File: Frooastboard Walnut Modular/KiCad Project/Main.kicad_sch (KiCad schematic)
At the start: 322 parts, among them J12 Conn_01x16, J13 Conn_01x06, J14 Conn_01x06, J15 F Row, J16 F Row USB, J17 Numpad, M2 Frooastboard_MM2040

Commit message: almost finish schematic
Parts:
- removed D? (x102): RGB_LED_6_Pin, Frooastboard Footprints:Everlight 99-235, symbol Frooastboard Symbols:RGB_LED_6_Pin
- removed J12: Conn_01x16, symbol Connector_Generic:Conn_01x16
- removed J13, J14: Conn_01x06, symbol Connector_Generic:Conn_01x06
- removed J?: Conn_01x16_Male, symbol Connector:Conn_01x16_Male
- removed J?: Conn_01x15_Male, symbol Connector:Conn_01x15_Male
- removed J? (x2): Conn_01x06_Male, symbol Connector:Conn_01x06_Male
- removed R23, R24: 27R, Resistor_SMD:R_0805_2012Metric, symbol Device:R_Small
- gave numbers to parts that had none: 5
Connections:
- net CS1: now also M2.13 (CS1)
- net CS10: now also M2.22 (CS10)
- net CS11: now also M2.23 (CS11)
- net CS12: now also M2.24 (CS12)
- net CS13: now also M2.25 (CS13)
- net CS14: now also M2.26 (CS14)
- net CS15: now also M2.27 (CS15)
- net CS16: now also M2.28 (CS16)
- net CS2: now also M2.14 (CS2)
- net CS3: now also M2.15 (CS3)
- net CS4: now also M2.16 (CS4)
- net CS5: now also M2.17 (CS5)
- net CS6: now also M2.18 (CS6)
- net CS7: now also M2.19 (CS7)
- net CS8: now also M2.20 (CS8)
- net CS9: now also M2.21 (CS9)
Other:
- moved on the sheet: C38, D113, D114, D115, D116, D117, D122, D123, D124, D125, D126, D127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

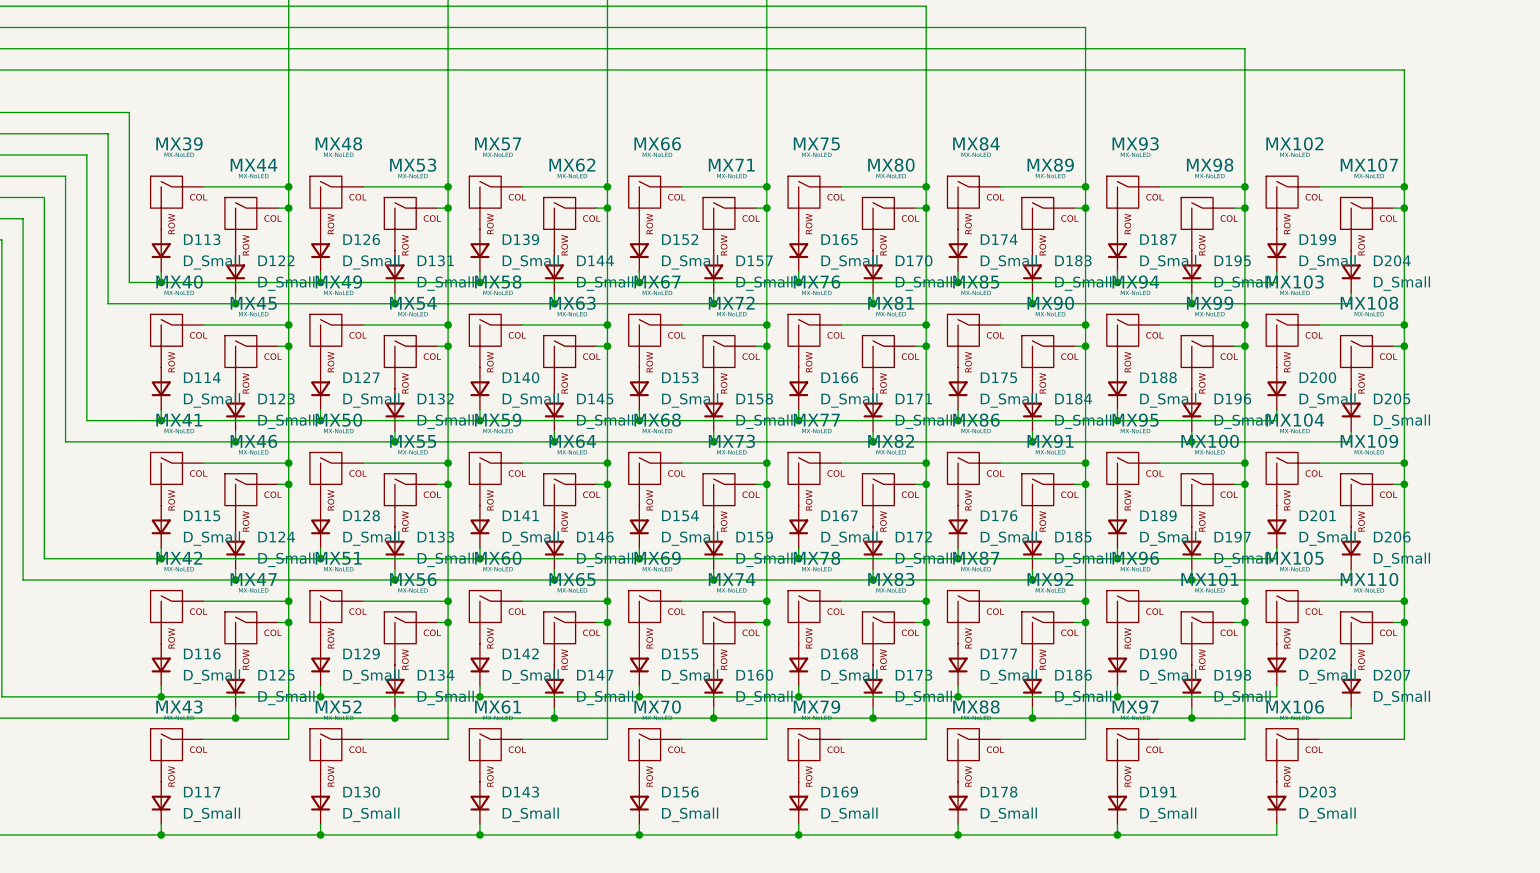
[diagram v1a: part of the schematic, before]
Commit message: do some stuff
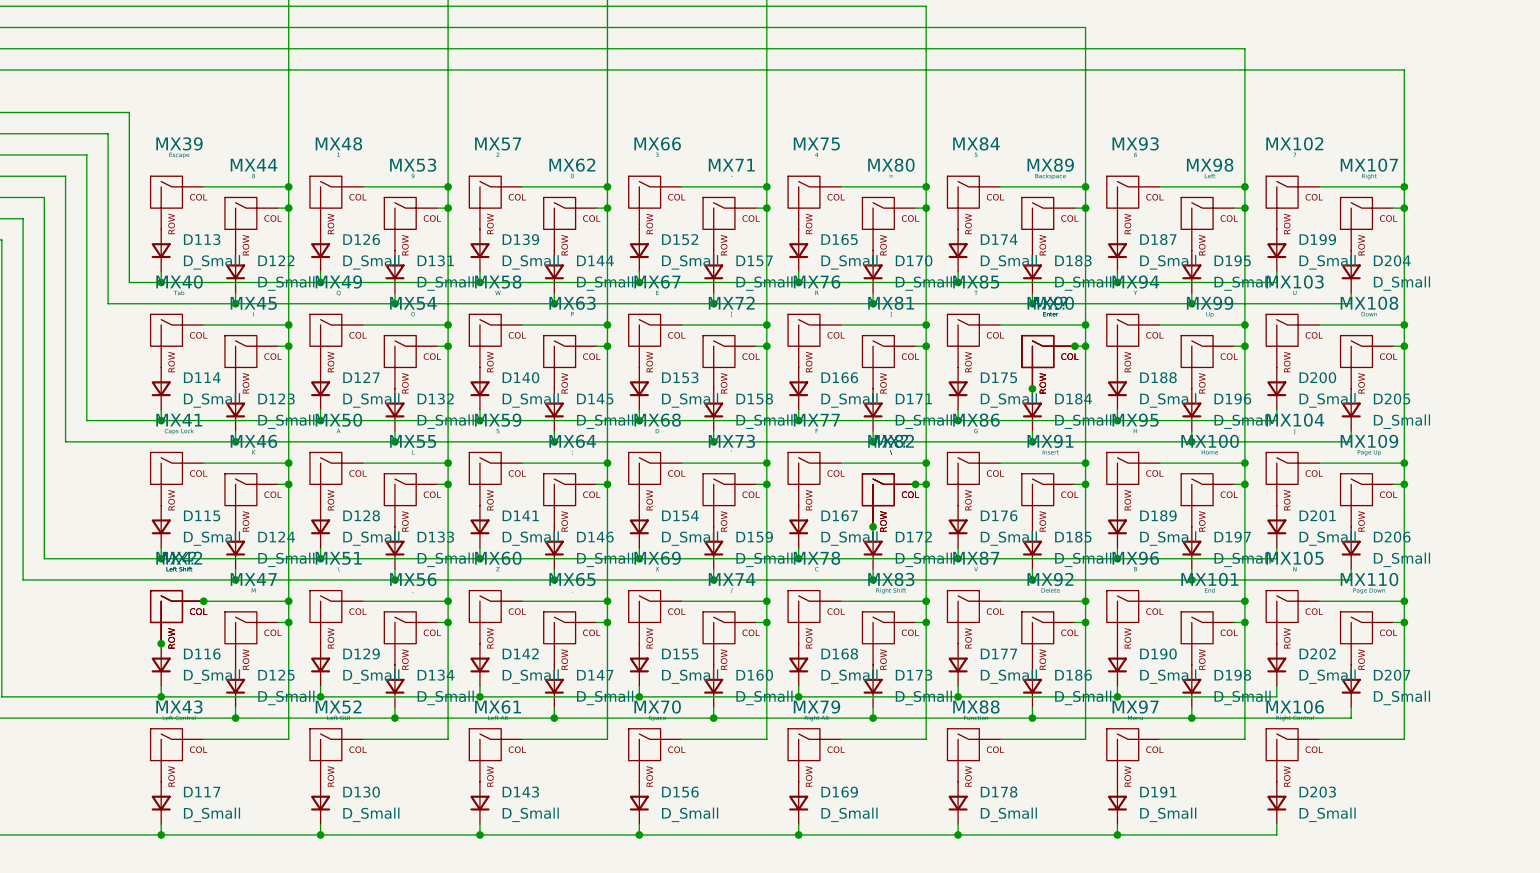
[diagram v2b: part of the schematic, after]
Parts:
- added MX?: Enter, symbol MX_Alps_Hybrid:MX-NoLED
- added MX?: Left Shift, symbol MX_Alps_Hybrid:MX-NoLED
- added MX?: \, symbol MX_Alps_Hybrid:MX-NoLED
- MX100: value MX-NoLED -> Home
- MX101: value MX-NoLED -> End
- MX102: value MX-NoLED -> 7
- MX103: value MX-NoLED -> U
- MX104: value MX-NoLED -> J
- MX105: value MX-NoLED -> N
- MX106: value MX-NoLED -> Right Control
- MX107: value MX-NoLED -> Right
- MX108: value MX-NoLED -> Down
- MX109: value MX-NoLED -> Page Up
- MX110: value MX-NoLED -> Page Down
- MX39: value MX-NoLED -> Escape
- MX40: value MX-NoLED -> Tab
- MX41: value MX-NoLED -> Caps Lock
- MX42: value MX-NoLED -> Left Shift
- MX43: value MX-NoLED -> Left Control
- MX44: value MX-NoLED -> 8
- MX45: value MX-NoLED -> I
- MX46: value MX-NoLED -> K
- MX47: value MX-NoLED -> M
- MX48: value MX-NoLED -> 1
- MX49: value MX-NoLED -> Q
- MX50: value MX-NoLED -> A
- MX51, MX82: value MX-NoLED -> \
- MX52: value MX-NoLED -> Left GUI
- MX53: value MX-NoLED -> 9
- MX54: value MX-NoLED -> O
- MX55: value MX-NoLED -> L
- MX56: value MX-NoLED -> ,
- MX57: value MX-NoLED -> 2
- MX58: value MX-NoLED -> W
- MX59: value MX-NoLED -> S
- MX60: value MX-NoLED -> Z
- MX61: value MX-NoLED -> Left Alt
- MX62: value MX-NoLED -> 0
- MX63: value MX-NoLED -> P
- MX64: value MX-NoLED -> ;
- MX65: value MX-NoLED -> .
- MX66: value MX-NoLED -> 3
- MX67: value MX-NoLED -> E
- MX68: value MX-NoLED -> D
- MX69: value MX-NoLED -> X
- MX70: value MX-NoLED -> Space
- MX71: value MX-NoLED -> -
- MX72: value MX-NoLED -> [
- MX73: value MX-NoLED -> '
- MX74: value MX-NoLED -> /
- MX75: value MX-NoLED -> 4
- MX76: value MX-NoLED -> R
- MX77: value MX-NoLED -> F
- MX78: value MX-NoLED -> C
- MX79: value MX-NoLED -> Right Alt
- MX80: value MX-NoLED -> =
- MX81: value MX-NoLED -> ]
- MX83: value MX-NoLED -> Right Shift
- MX84: value MX-NoLED -> 5
- MX85: value MX-NoLED -> T
- MX86: value MX-NoLED -> G
- MX87: value MX-NoLED -> V
- MX88: value MX-NoLED -> Function
- MX89: value MX-NoLED -> Backspace
- MX90: value MX-NoLED -> Enter
- MX91: value MX-NoLED -> Insert
- MX92: value MX-NoLED -> Delete
- MX93: value MX-NoLED -> 6
- MX94: value MX-NoLED -> Y
- MX95: value MX-NoLED -> H
- MX96: value MX-NoLED -> B
- MX97: value MX-NoLED -> Menu
- MX98: value MX-NoLED -> Left
- MX99: value MX-NoLED -> Up
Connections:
- net COL0: now also MX?.1 (COL)
- net COL4: now also MX?.1 (COL)
- net COL5: now also MX?.1 (COL)
- net at D116.2 (A), MX42.2 (ROW): now also MX?.2 (ROW)
- net at D184.2 (A), MX90.2 (ROW): now also MX?.2 (ROW)
- net at D172.2 (A), MX82.2 (ROW): now also MX?.2 (ROW)

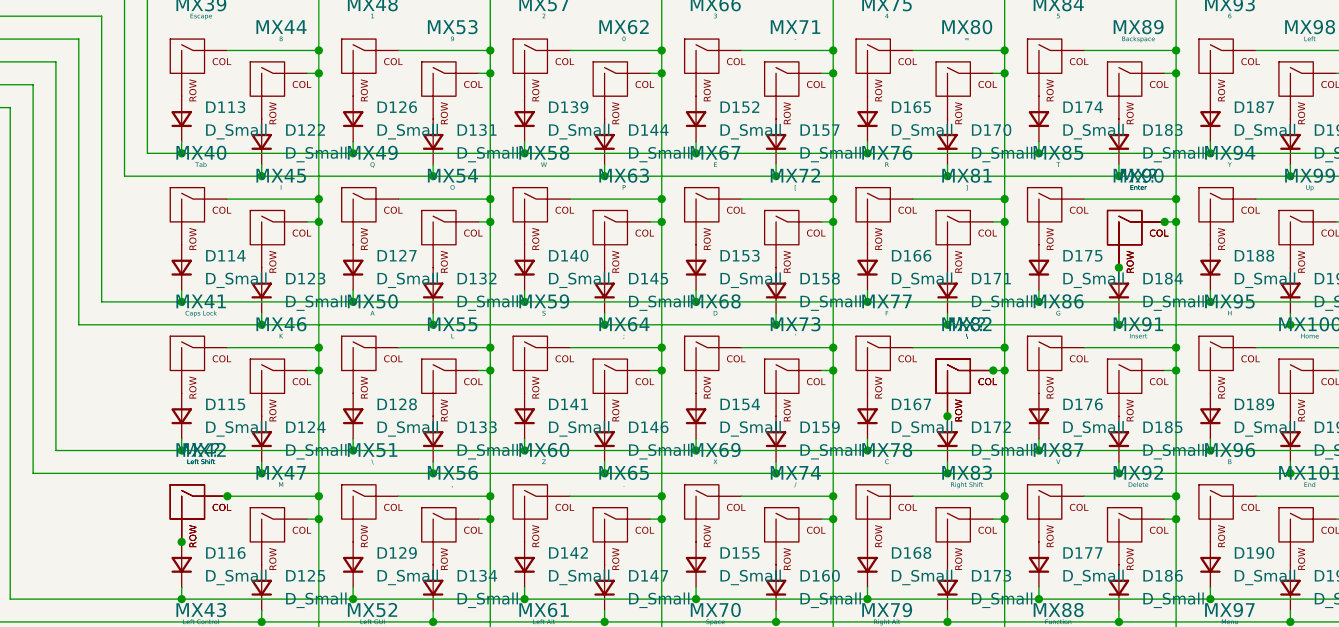
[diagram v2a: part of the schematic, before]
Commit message: before nrf52810
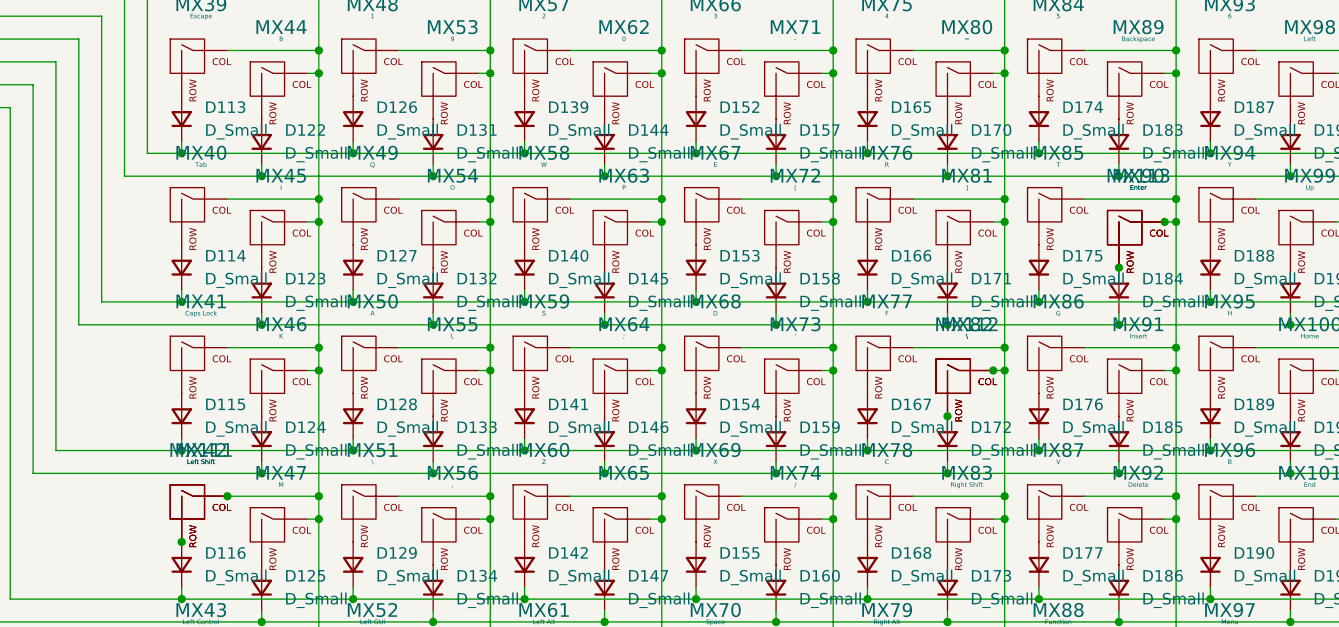
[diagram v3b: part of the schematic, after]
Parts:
- gave numbers to parts that had none: 3
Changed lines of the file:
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@@
   (symbol (lib_id "MX_Alps_Hybrid:MX-NoLED") (at 163.83 204.47 0) (unit 1)
     (in_bom yes) (on_board yes) (fields_autoplaced)
-    (property "Reference" "MX?" (id 0) (at 164.7156 198.12 0)
+    (property "Reference" "MX113" (id 0) (at 164.7156 198.12 0)
       (effects (font (size 1.524 1.524)))
     )
@@
   (symbol (lib_id "MX_Alps_Hybrid:MX-NoLED") (at 59.69 234.95 0) (unit 1)
     (in_bom yes) (on_board yes) (fields_autoplaced)
-    (property "Reference" "MX?" (id 0) (at 60.5756 228.6 0)
+    (property "Reference" "MX111" (id 0) (at 60.5756 228.6 0)
       (effects (font (size 1.524 1.524)))
     )
@@
   (symbol (lib_id "MX_Alps_Hybrid:MX-NoLED") (at 144.78 220.98 0) (unit 1)
     (in_bom yes) (on_board yes) (fields_autoplaced)
-    (property "Reference" "MX?" (id 0) (at 145.6656 214.63 0)
-      (effects (font (size 1.524 1.524)))
-    )
+    (property "Reference" "MX112" (id 0) (at 145.6656 214.63 0)
+      (effects (font (size 1.524 1.524)))
+    )
